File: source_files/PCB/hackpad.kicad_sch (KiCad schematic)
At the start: 18 parts, among them J1 Conn_01x04, SW1 SW_Push, SW2 SW_Push, SW3 SW_Push, SW4 SW_Push, SW5 SW_Push, SW6 SW_Push, SW7 SW_Push, SW8 RotaryEncoder_Switch, U1 MOUDLE-SEEEDUINO-XIAO

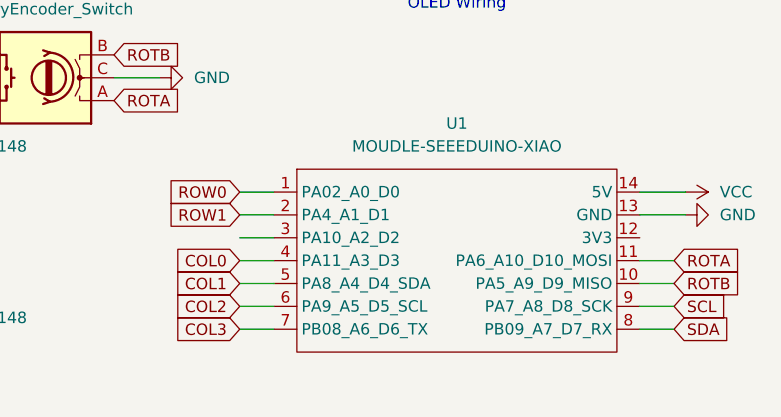
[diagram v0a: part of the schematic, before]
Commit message: Add files via upload
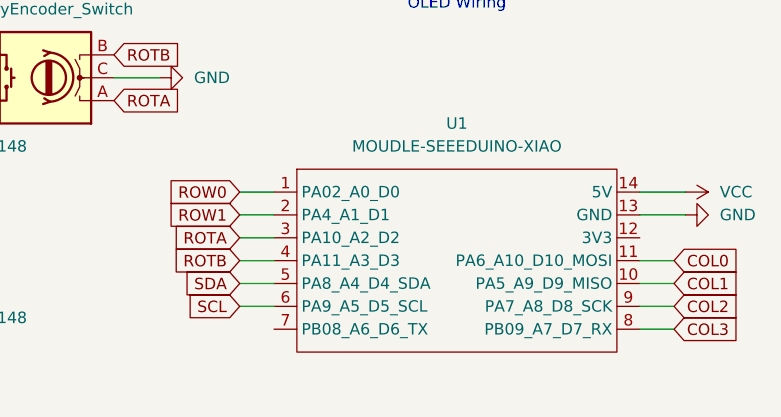
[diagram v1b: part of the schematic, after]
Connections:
- net COL0: now also U1.11 (PA6_A10_D10_MOSI); no longer U1.4 (PA11_A3_D3)
- net COL1: now also U1.10 (PA5_A9_D9_MISO); no longer U1.5 (PA8_A4_D4_SDA)
- net COL2: now also U1.9 (PA7_A8_D8_SCK); no longer U1.6 (PA9_A5_D5_SCL)
- net COL3: now also U1.8 (PB09_A7_D7_RX); no longer U1.7 (PB08_A6_D6_TX)
- net ROTA: now also U1.3 (PA10_A2_D2); no longer U1.11 (PA6_A10_D10_MOSI)
- net ROTB: now also U1.4 (PA11_A3_D3); no longer U1.10 (PA5_A9_D9_MISO)
- net SCL: now also U1.6 (PA9_A5_D5_SCL); no longer U1.9 (PA7_A8_D8_SCK)
- net SDA: now also U1.5 (PA8_A4_D4_SDA); no longer U1.8 (PB09_A7_D7_RX)
